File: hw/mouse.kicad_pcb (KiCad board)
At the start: 2 copper layers, 73.7 x 33 mm, 26 parts, among them J1 JUMPER2, J2 JUMPER2, J3 CONN-ISP-6, J4 CONN_2X1, J5 CONN_5X1, J6 CONN_3X1, J8 CONN_4X2, J9 CONN_5X2, U1 12MHz, U2 ATtiny2313-20PU, U3 MAX232N

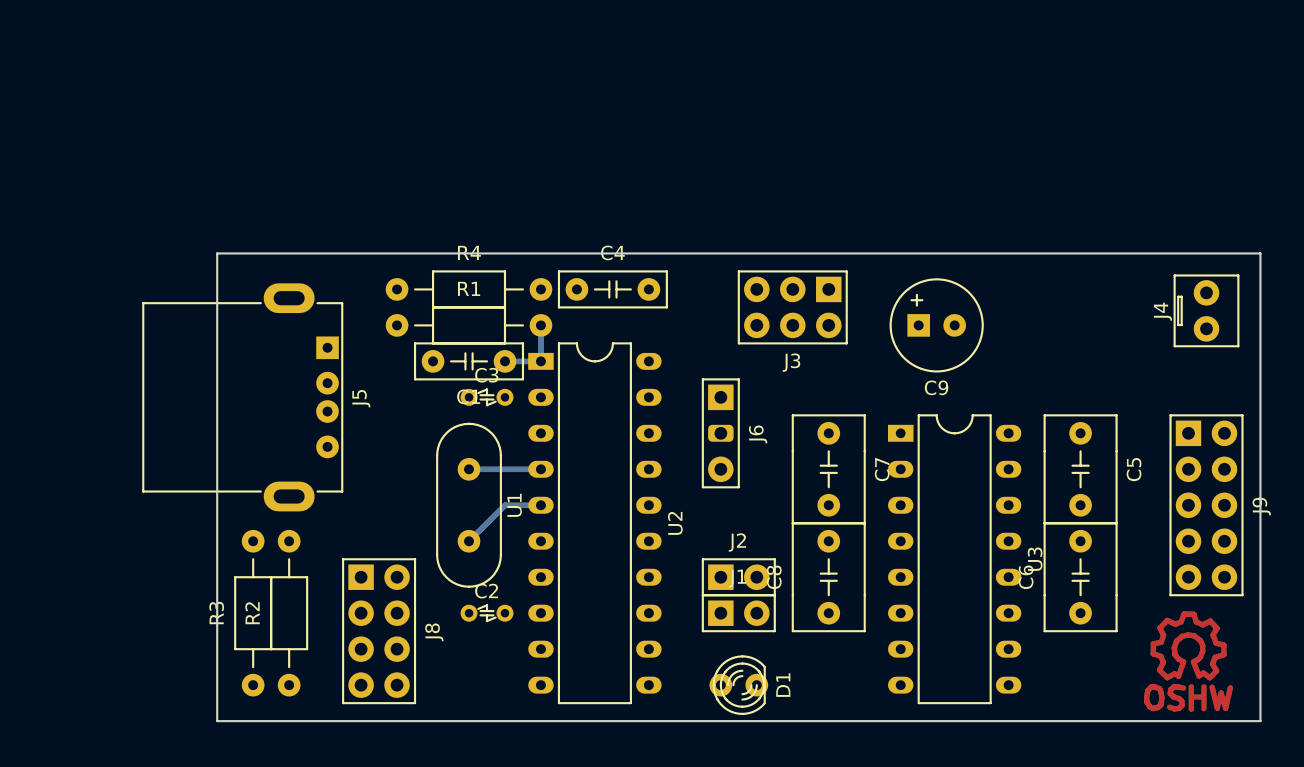
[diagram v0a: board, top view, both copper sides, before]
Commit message: add Kicad PCB
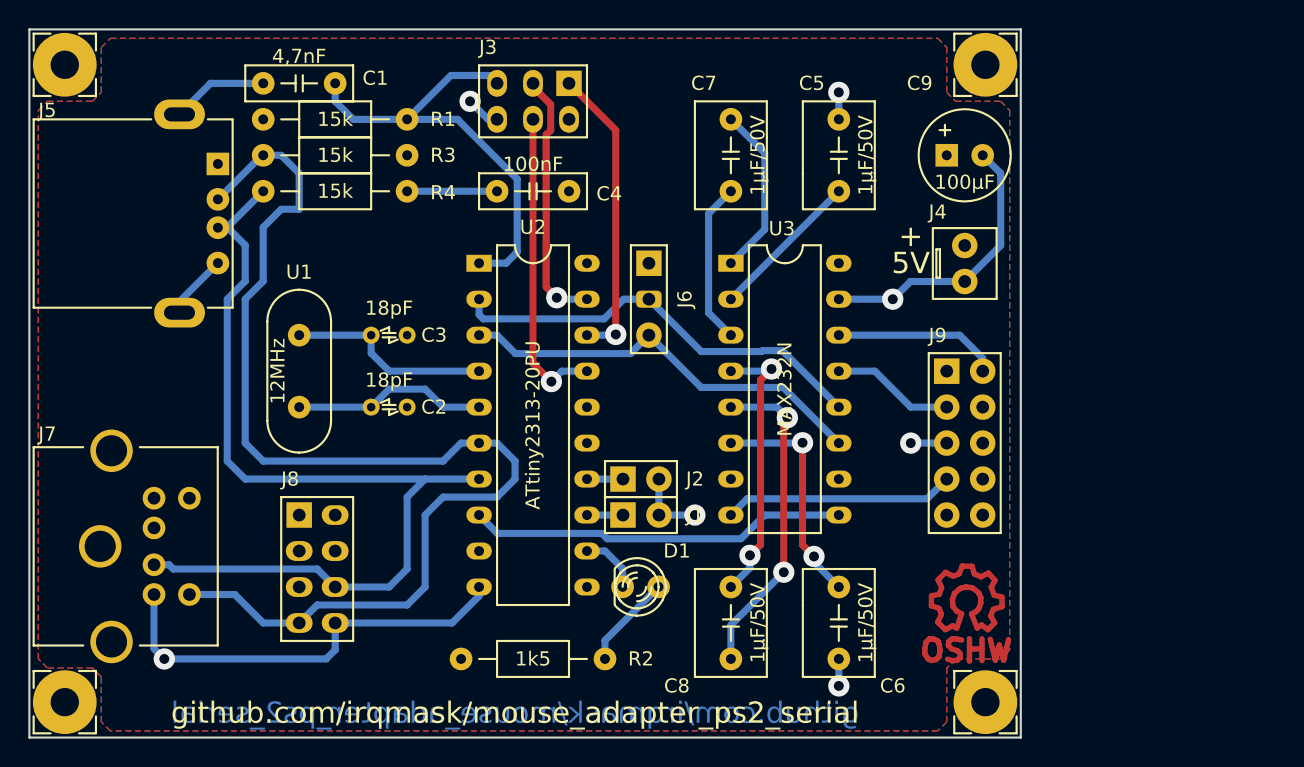
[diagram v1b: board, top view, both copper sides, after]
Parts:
- added HOLE_2.5mm: VAL**, Mechanical:HOLE_2mm, F.Cu at (101.0, 115.5)
- added HOLE_2.5mm: VAL**, Mechanical:HOLE_2mm, F.Cu at (166.0, 115.5)
- added HOLE_2.5mm: VAL**, Mechanical:HOLE_2mm, F.Cu at (166.0, 70.5)
- added HOLE_2.5mm: VAL**, Mechanical:HOLE_2mm, F.Cu at (101.0, 70.5)
- added J7: Mini-DIN-6, Connector_Miscelleaneus:MiniDIN_6pole, F.Cu at (98.8, 104.5)
- C5, C6, C7, C8: value 1,0µF/50V (MKS2) -> 1µF/50V
- D1: value LED 3mm green, 2mA, 1,9V -> LED gr 2mA, 1,9V
- J1: value JUMPER2 -> J1
- J2: value JUMPER2 -> J2
- moved R3 37.4 mm to (115.0, 76.9), turned to 0 degrees
- moved C5 28.0 mm to (155.7, 76.9), turned to 270 degrees
- moved J3 23.4 mm to (136.6, 71.8)
- moved C7 23.2 mm to (148.0, 76.9)
- moved C1 23.0 mm to (117.5, 71.8)
- moved J9 17.6 mm to (163.3, 92.1)
- moved J4 17.4 mm to (164.5, 85.8)
- moved C6 17.4 mm to (155.7, 109.9), turned to 90 degrees
- moved R1 17.3 mm to (115.0, 74.3)
- moved U3 17.0 mm to (148.0, 84.5)
- moved C2 16.1 mm to (125.2, 94.7)
- moved LOGO1 16.0 mm to (164.7, 108.4)
- moved U1 15.3 mm to (117.5, 92.1)
- moved J5 15.1 mm to (109.1, 81.0)
- moved R2 12.3 mm to (129.0, 112.5), turned to 0 degrees
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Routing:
- net GND: track 0.00 -> 82.2 mm, vias 0 -> 7
- net /MCLK: track 0.00 -> 81.8 mm
- net /MDTA: track 0.00 -> 66.7 mm
- net /RXD: track 0.00 -> 30.4 mm
- net /TXD: track 0.00 -> 29.6 mm
- net /RESET: track 5.08 -> 32.4 mm
- net /RTS: track 0.00 -> 26.8 mm
- net Net-(C8-Pad2): track 0.00 -> 23.0 mm, vias 0 -> 2
- net /MOSI: track 0.00 -> 21.9 mm, vias 0 -> 1
- net /MISO: track 0.00 -> 21.1 mm, vias 0 -> 1
- net Net-(C8-Pad1): track 0.00 -> 19.6 mm, vias 0 -> 2
- net /SCL: track 0.00 -> 18.3 mm, vias 0 -> 1
- net Net-(C6-Pad2): track 0.00 -> 16.3 mm, vias 0 -> 2
- net Net-(J9-Pad7): track 0.00 -> 16.3 mm
- net Net-(C7-Pad2): track 0.00 -> 12.1 mm
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- added copper zone on B.Cu, net +5V
- added copper zone on F.Cu, net GND
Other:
- board size 73.7 x 33 mm -> 70 x 50 mm
- net class Default: trace_width 0.4 -> 0.5; via_dia 1.2 -> 1.5
- rule trace_min: 0.2 -> 0.5
- rule via_min_size: 0.4 -> 0.6
- board text added: "+"
- board text added: "5V"
- board text added: "github.com/irqmask/mouse_adapter_ps2_serial"
